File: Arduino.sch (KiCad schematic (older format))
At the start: 0 parts

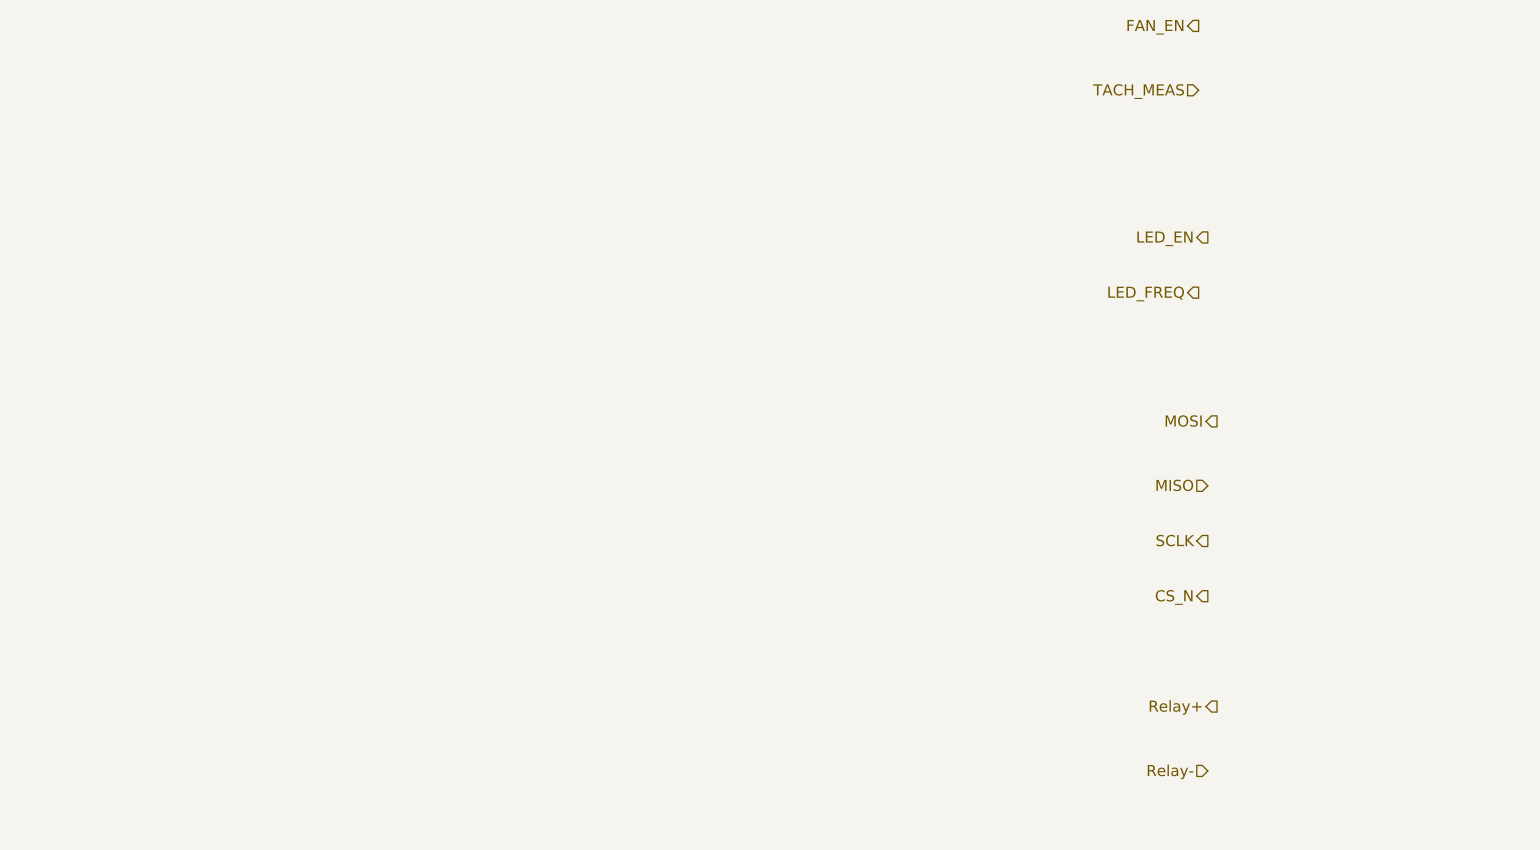
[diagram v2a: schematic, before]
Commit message: Arduino
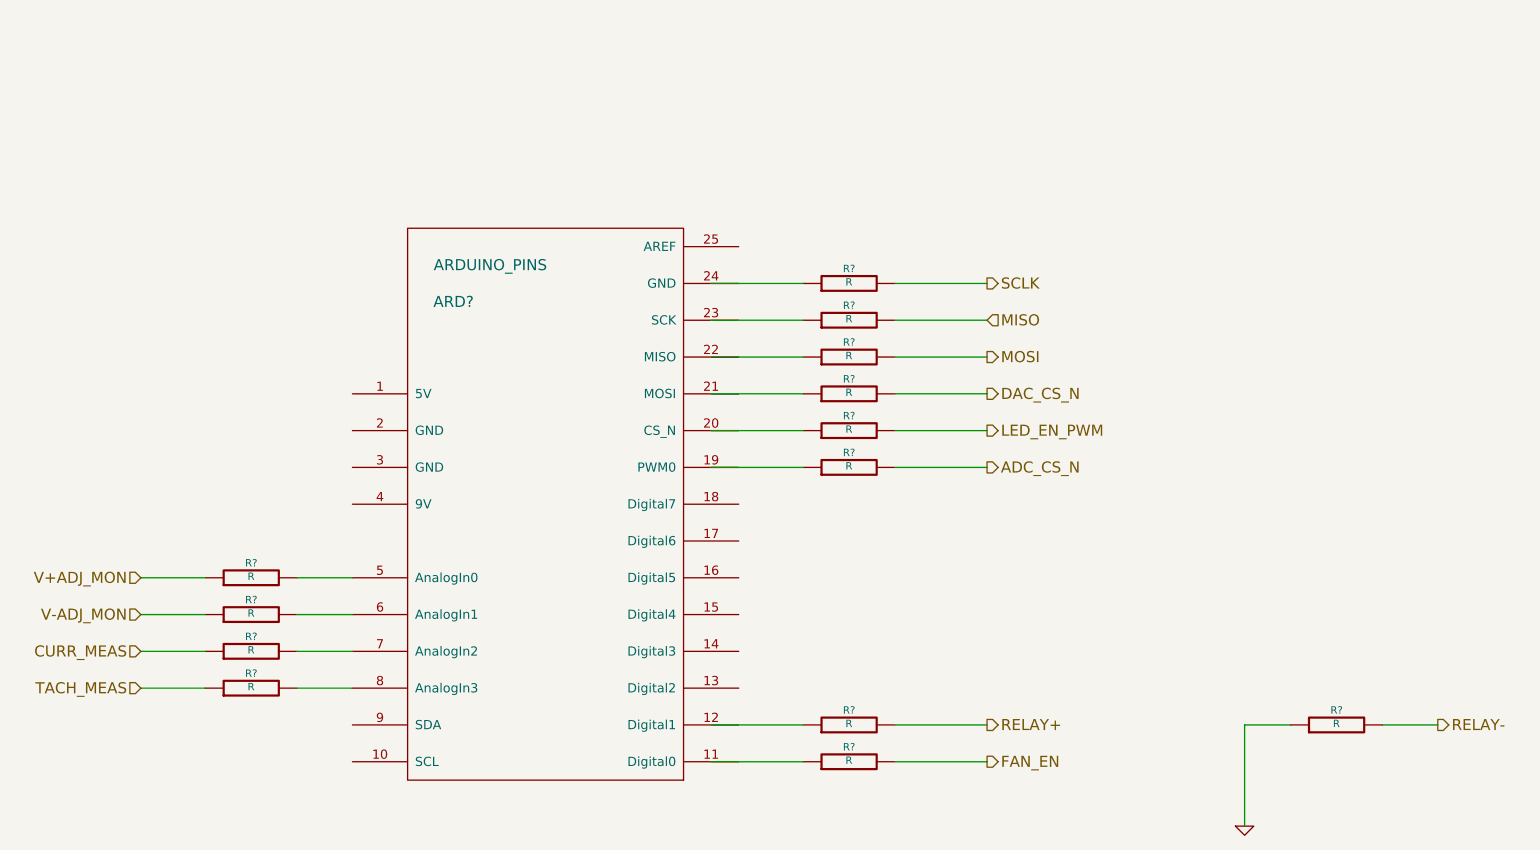
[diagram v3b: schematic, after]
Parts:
- added ARD?: ARDUINO_PINS, ~, symbol ARDUINO_PINS
- added R? (x13): R, ~, symbol R
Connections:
- net labels added: ADC_CS_N, CURR_MEAS, DAC_CS_N, GND, LED_EN_PWM, RELAY+, RELAY-, V+ADJ_MON, V-ADJ_MON
- net labels removed: CS_N, LED_EN, LED_FREQ, Relay+, Relay-
- wire segments 0 -> 27
